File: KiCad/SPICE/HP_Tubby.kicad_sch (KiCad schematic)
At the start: 14 parts, among them U4 ${SIM.PARAMS}, U5 ${SIM.PARAMS}

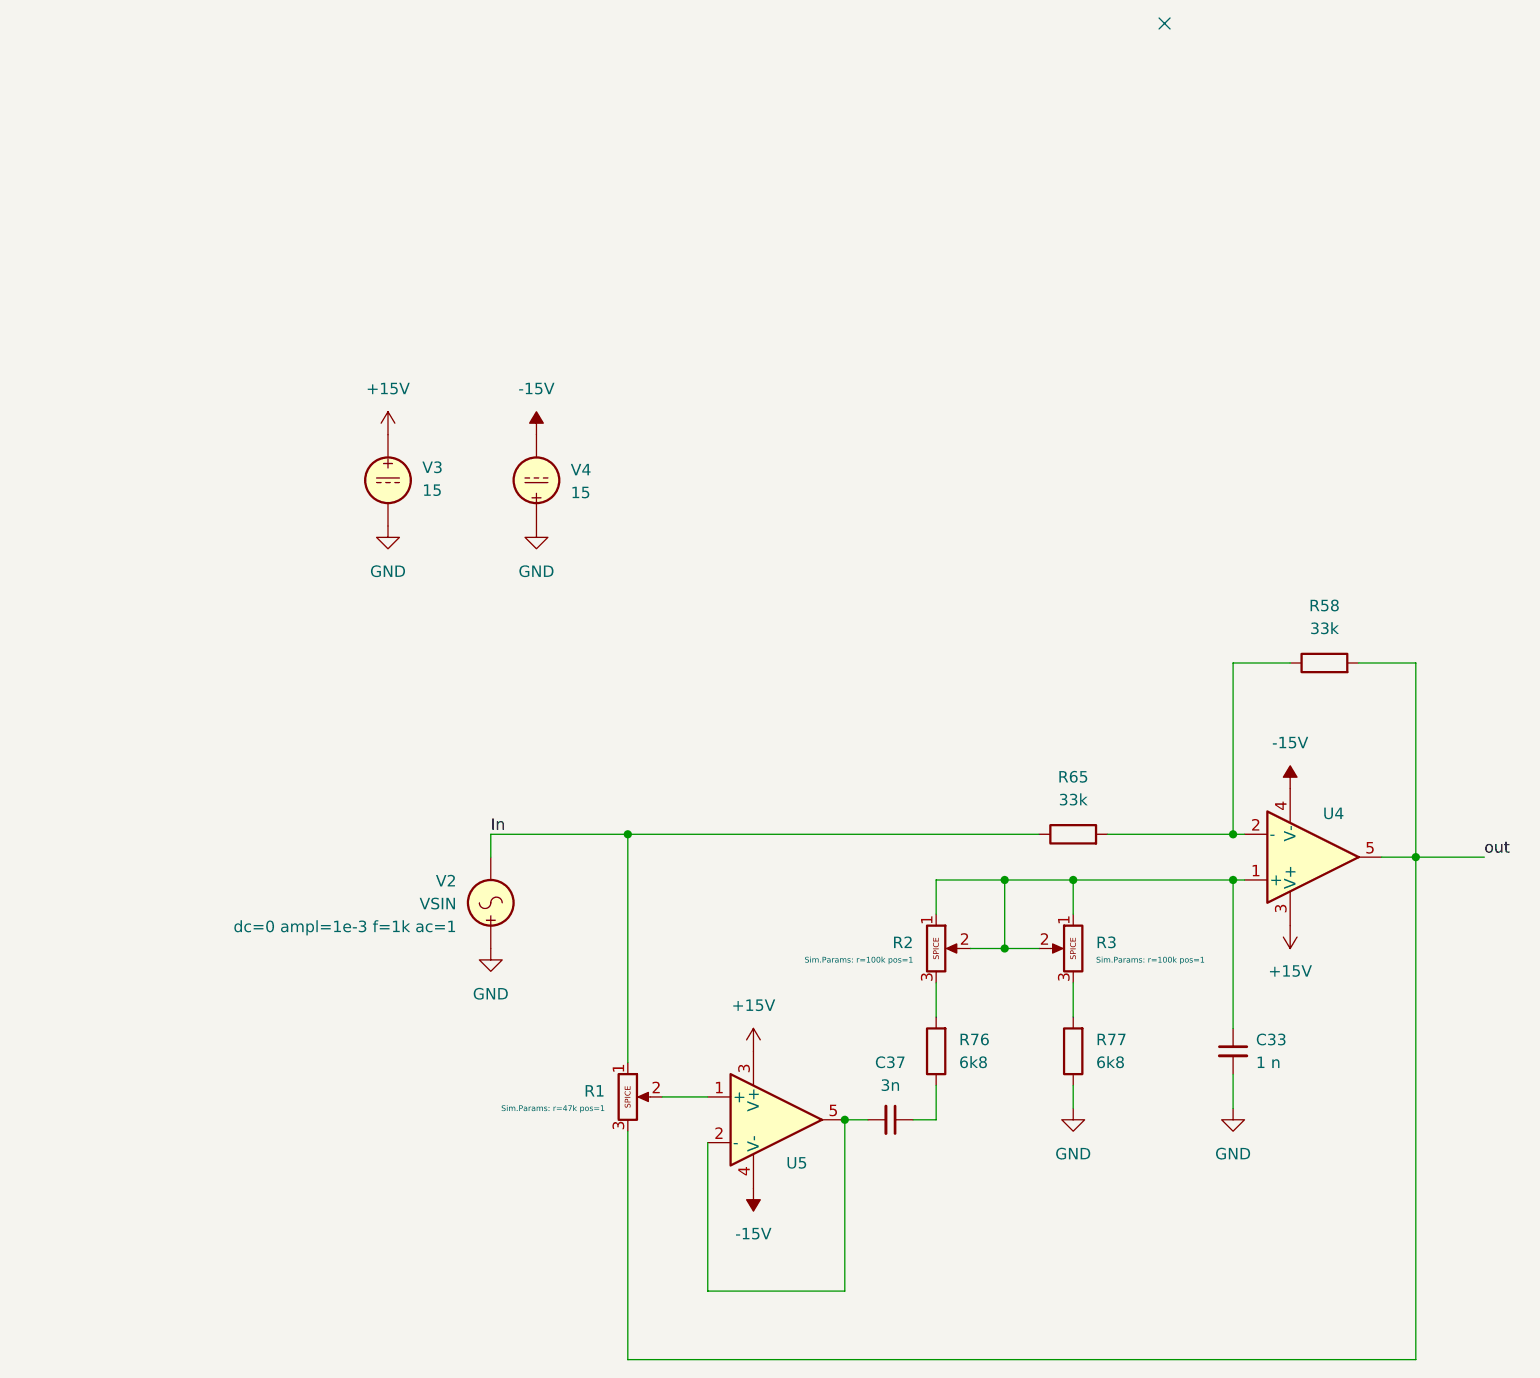
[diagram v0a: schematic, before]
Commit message: EQ Output Update
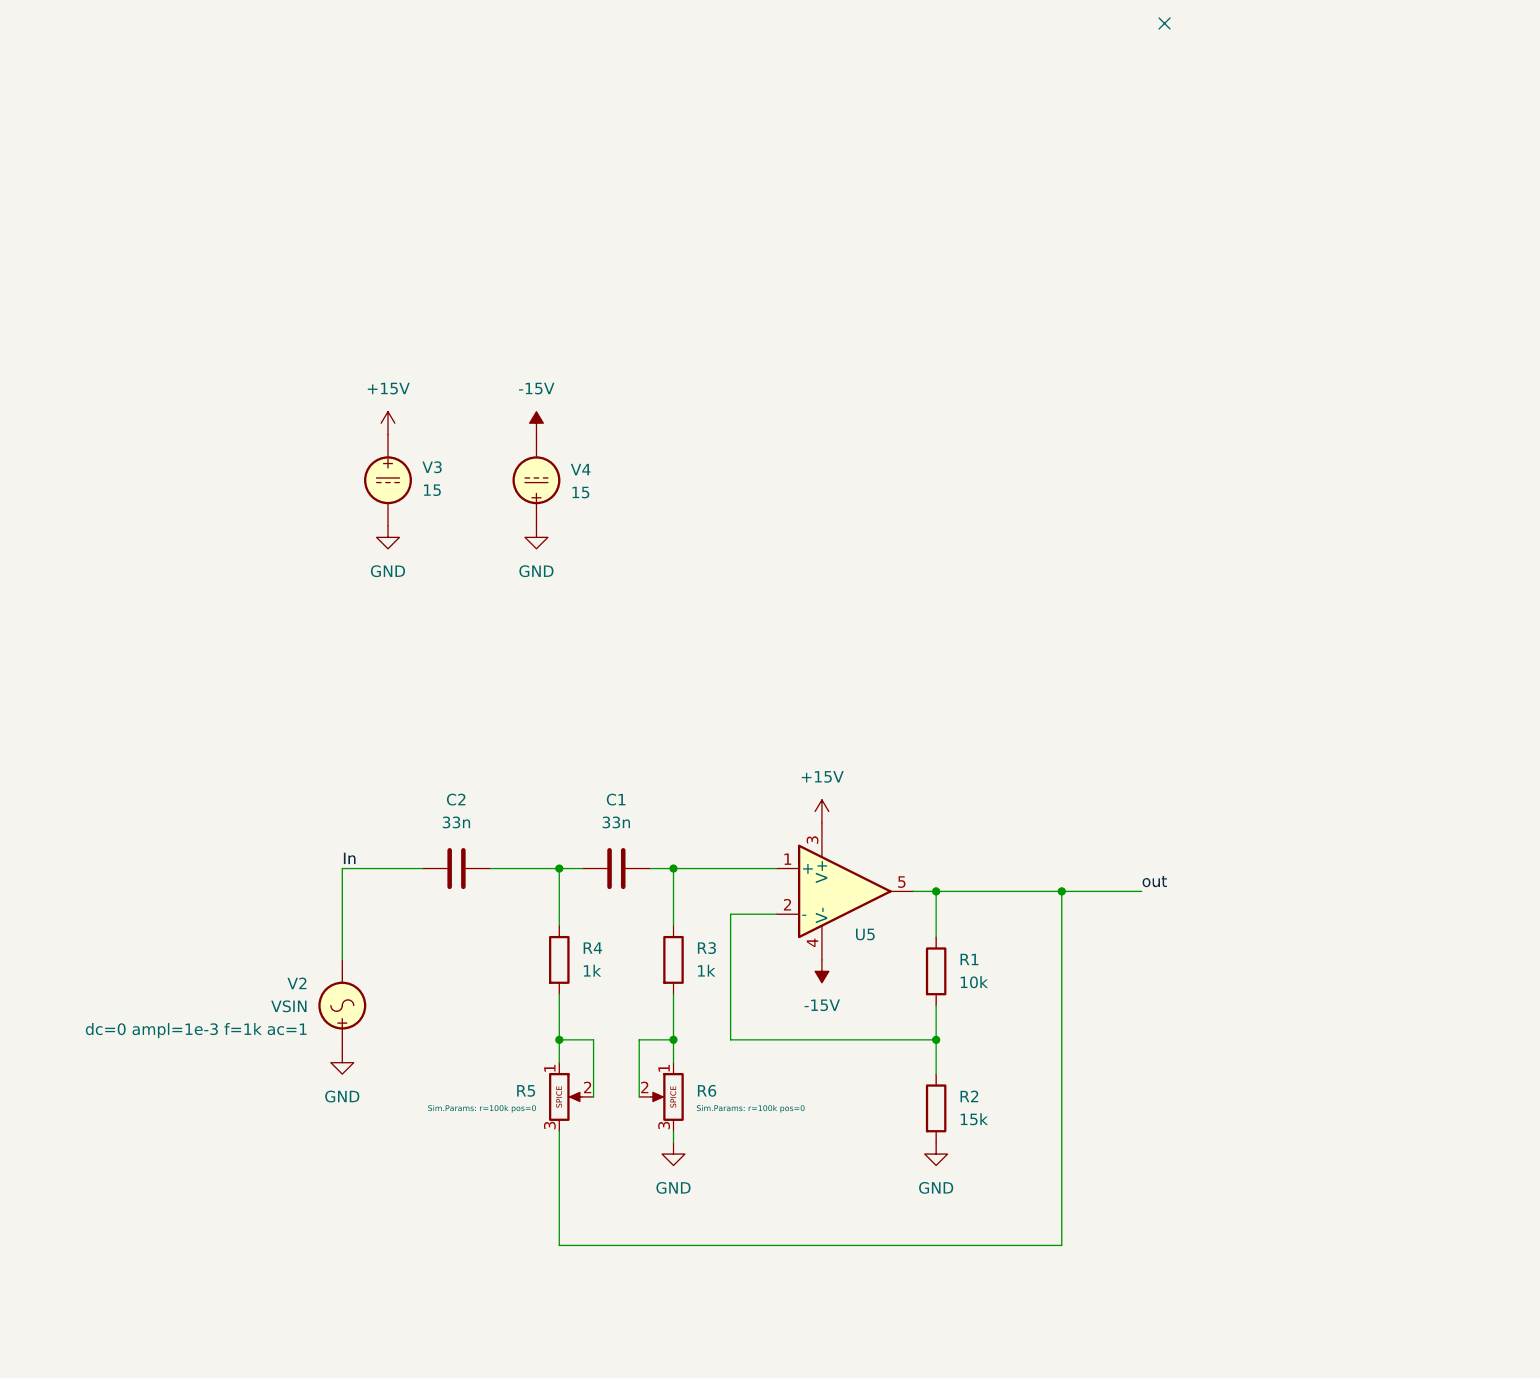
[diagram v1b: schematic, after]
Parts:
- removed C33: 1 n, Capacitor_SMD:C_0805_2012Metric_Pad1.18x1.45mm_HandSolder, symbol Device:C_Small
- removed C37: 3n, Capacitor_SMD:C_0805_2012Metric_Pad1.18x1.45mm_HandSolder, symbol Device:C_Small
- removed R1, R2, R3: Potentiometer, symbol Simulation_SPICE:Potentiometer
- removed R58, R65: 33k, Resistor_SMD:R_0805_2012Metric_Pad1.20x1.40mm_HandSolder, symbol Device:R
- removed R76, R77: 6k8, Resistor_SMD:R_0805_2012Metric_Pad1.20x1.40mm_HandSolder, symbol Device:R
- removed U4: ${SIM.PARAMS}, symbol Simulation_SPICE:OPAMP
- added C1, C2: 33n, symbol Device:C
- added R1: 10k, symbol Device:R
- added R2: 15k, symbol Device:R
- added R3, R4: 1k, symbol Device:R
- added R5, R6: Potentiometer, symbol Simulation_SPICE:Potentiometer
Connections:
- net GND: now also R2.2, R6.3
- net In: now also C2.1
- net out: now also U5.5, R1.1, R5.3
- net at U5.1 (+): now also C1.2, R3.1
- net at U5.2 (-): now also R1.2, R2.1; no longer U5.5
- new net: C1.1, C2.2, R4.1
- new net: R4.2, R5.1, R5.2
- new net: R3.2, R6.1, R6.2
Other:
- moved on the sheet: U5, V2
